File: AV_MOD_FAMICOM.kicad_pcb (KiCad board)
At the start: 2 copper layers, 85.1 x 45.7 mm, 13 parts, among them J1 USB-A-S-X-X-TH, J2 USB-A-S-X-X-TH, J3 Conn_01x02_Male, J5 Conn_01x07, Q1 Q_PNP_CBE, Q2 Q_NPN_CBE

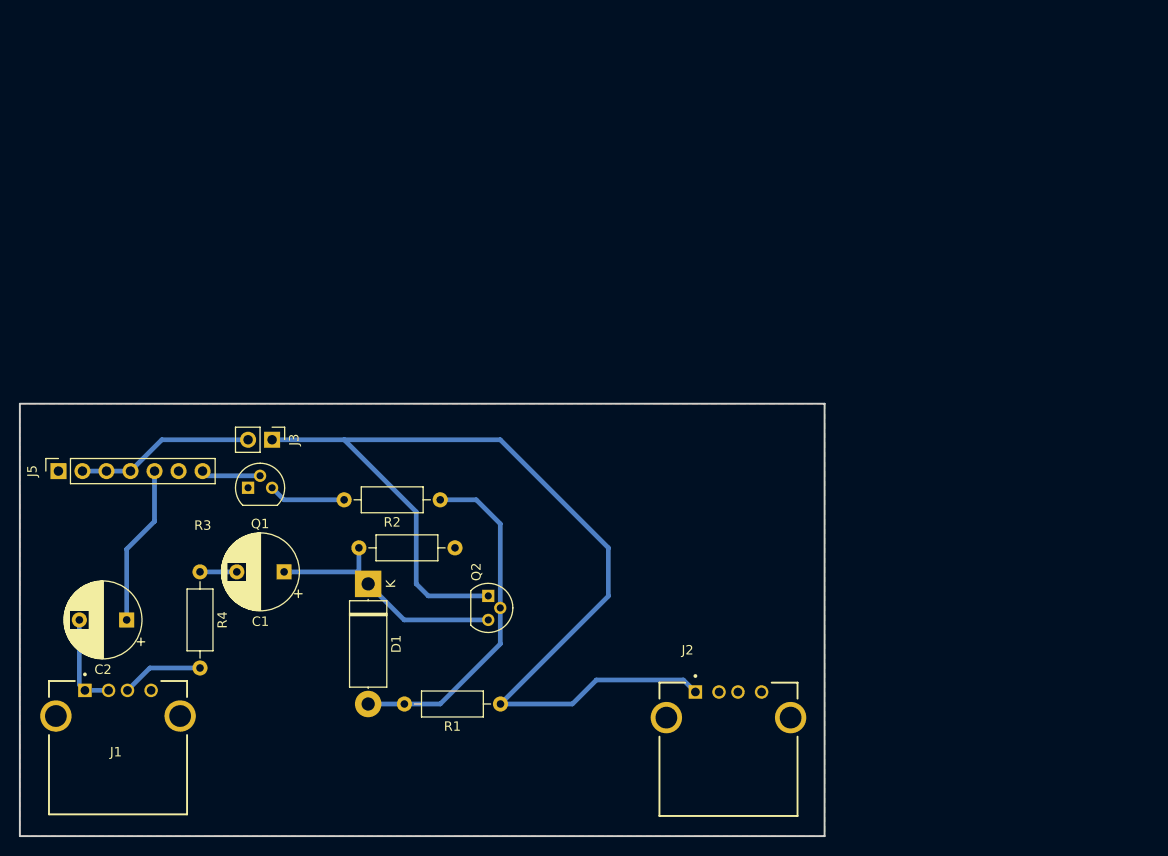
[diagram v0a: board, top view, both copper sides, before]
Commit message: Add files via upload
New version of the board
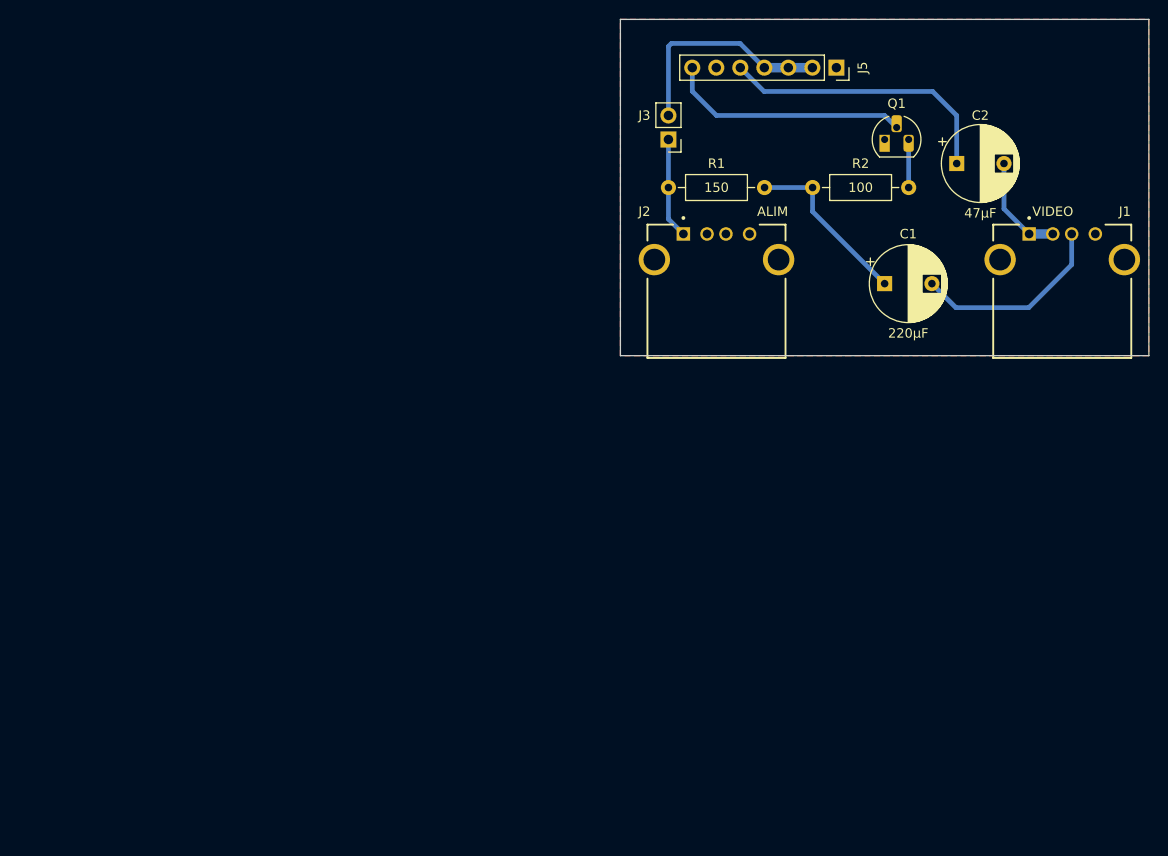
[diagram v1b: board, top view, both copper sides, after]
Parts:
- removed D1: DIODE, Diode_THT:D_5W_P12.70mm_Horizontal
- removed Q2: Q_NPN_CBE, Package_TO_SOT_THT:TO-92
- removed R3: 68, Resistor_THT:R_Axial_DIN0207_L6.3mm_D2.5mm_P10.16mm_Horizontal
- removed R4: 82?, Resistor_THT:R_Axial_DIN0207_L6.3mm_D2.5mm_P10.16mm_Horizontal
- Q1: footprint Package_TO_SOT_THT:TO-92 -> Package_TO_SOT_THT:TO-92L_HandSolder
- R1: value 2200 -> 150
- R2: value 220 -> 100
- moved J1 110.9 mm to (213.1, 58.4)
- moved C2 100.2 mm to (201.9, 48.3), turned to 0 degrees
- moved J5 92.7 mm to (189.2, 38.1), turned to -90 degrees
- moved Q1 76.7 mm to (194.3, 45.7)
- moved C1 70.4 mm to (194.3, 61.0), turned to 0 degrees
- moved R1 57.4 mm to (171.4, 50.8), turned to 0 degrees
- moved J3 52.6 mm to (171.4, 45.7), turned to 180 degrees
- moved R2 51.4 mm to (186.7, 50.8), turned to 0 degrees
- moved J2 48.4 mm to (176.5, 58.4)
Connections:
- C1 pad 2: Net-(C1-Pad2) -> VIDEO OUT
- J1 pad S1: Net-(J1-PadS1) -> GNDREF
- J1 pad S2: Net-(J1-PadS1) -> GNDREF
- J2 pad S1: Net-(J2-PadS1) -> GNDREF
- J2 pad S2: Net-(J2-PadS1) -> GNDREF
- R1 pad 2: Net-(D1-Pad2) -> Net-(C1-Pad1)
- R2 pad 1: Net-(D1-Pad2) -> Net-(C1-Pad1)
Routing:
- net +5V: track 110.3 -> 10.6 mm
- net Net-(D1-Pad2): track 36.7 -> 0.00 mm
- net VIDEO IN: track 6.29 -> 25.7 mm
- net AUDIO: track 17.0 -> 30.1 mm
- net VIDEO OUT: track 8.65 -> 21.0 mm
- net Net-(C1-Pad1): track 27.9 -> 18.4 mm
- net Net-(J3-Pad2): track 18.9 -> 23.7 mm
- net Net-(C1-Pad2): track 3.89 -> 0.00 mm
- net Net-(Q1-Pad3): track 8.15 -> 5.08 mm
- net AUDIO L: track 10.2 -> 11.1 mm
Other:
- board size 85.1 x 45.7 mm -> 55.9 x 35.6 mm
- board text added: "ALIM"
- board text added: "VIDEO"
